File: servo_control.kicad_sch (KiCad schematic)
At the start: 23 parts, among them U9 PCA9685PW

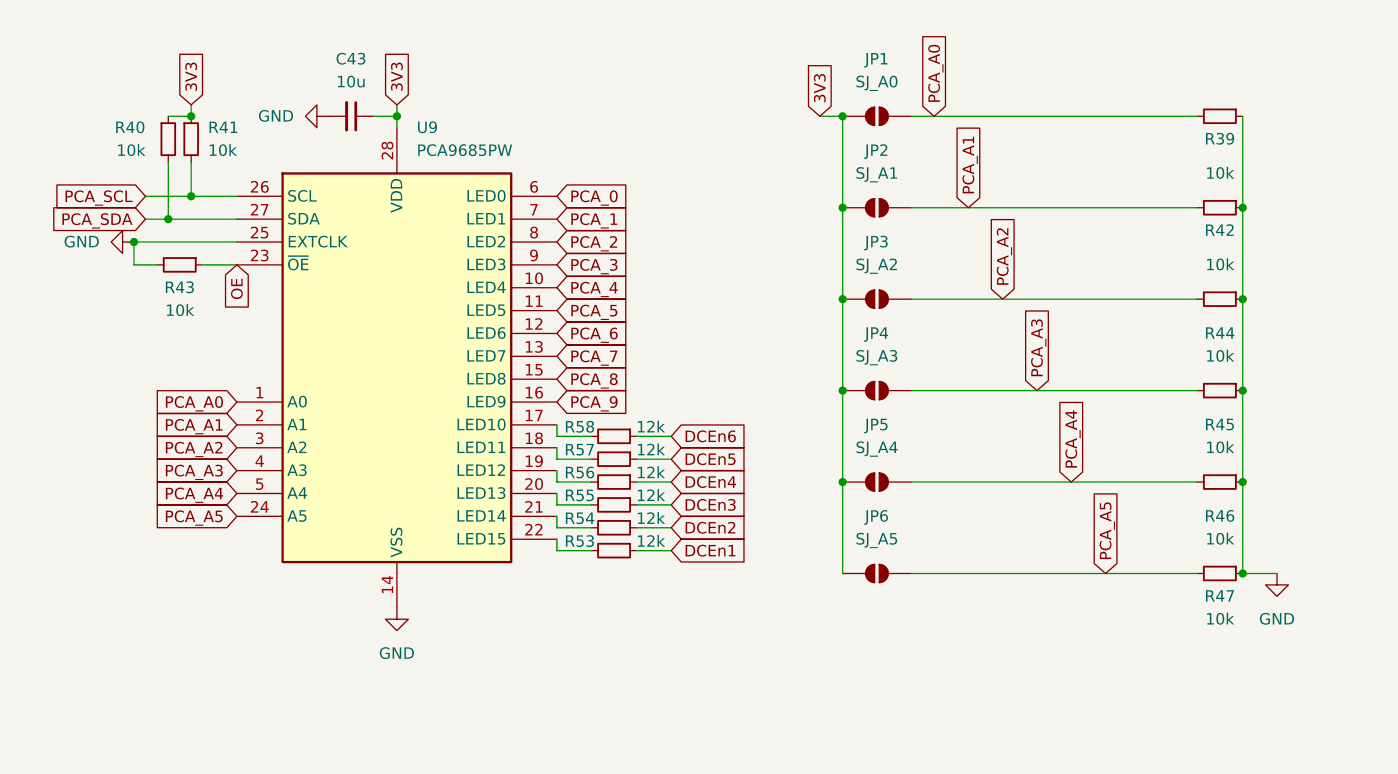
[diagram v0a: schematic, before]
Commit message: Visual Improvements
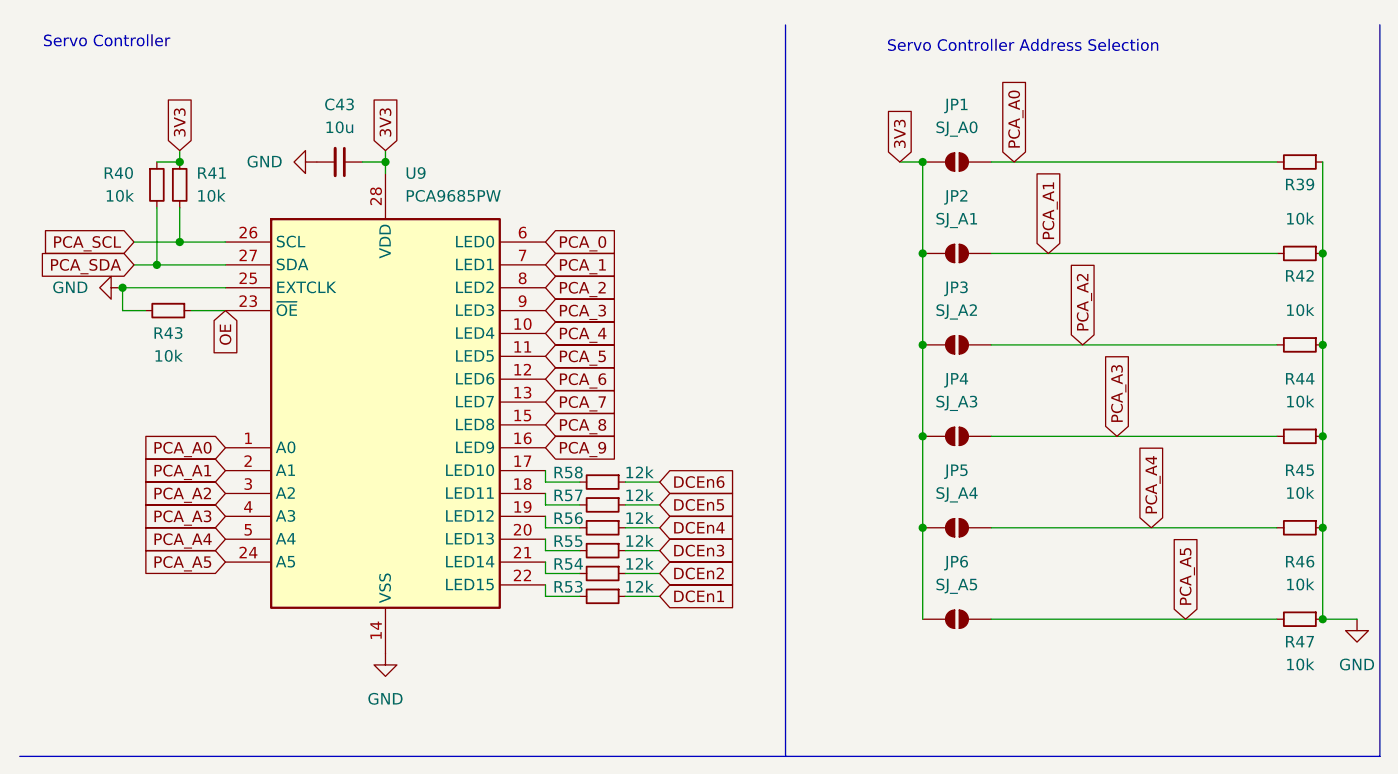
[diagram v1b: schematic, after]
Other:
- note added: "Servo Controller"
- note added: "Servo Controller Address Selection"
- moved on the sheet: C43, JP1, JP2, JP3, JP4, JP5, JP6, R39, R40, R41, R42, R43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

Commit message: schematic finished
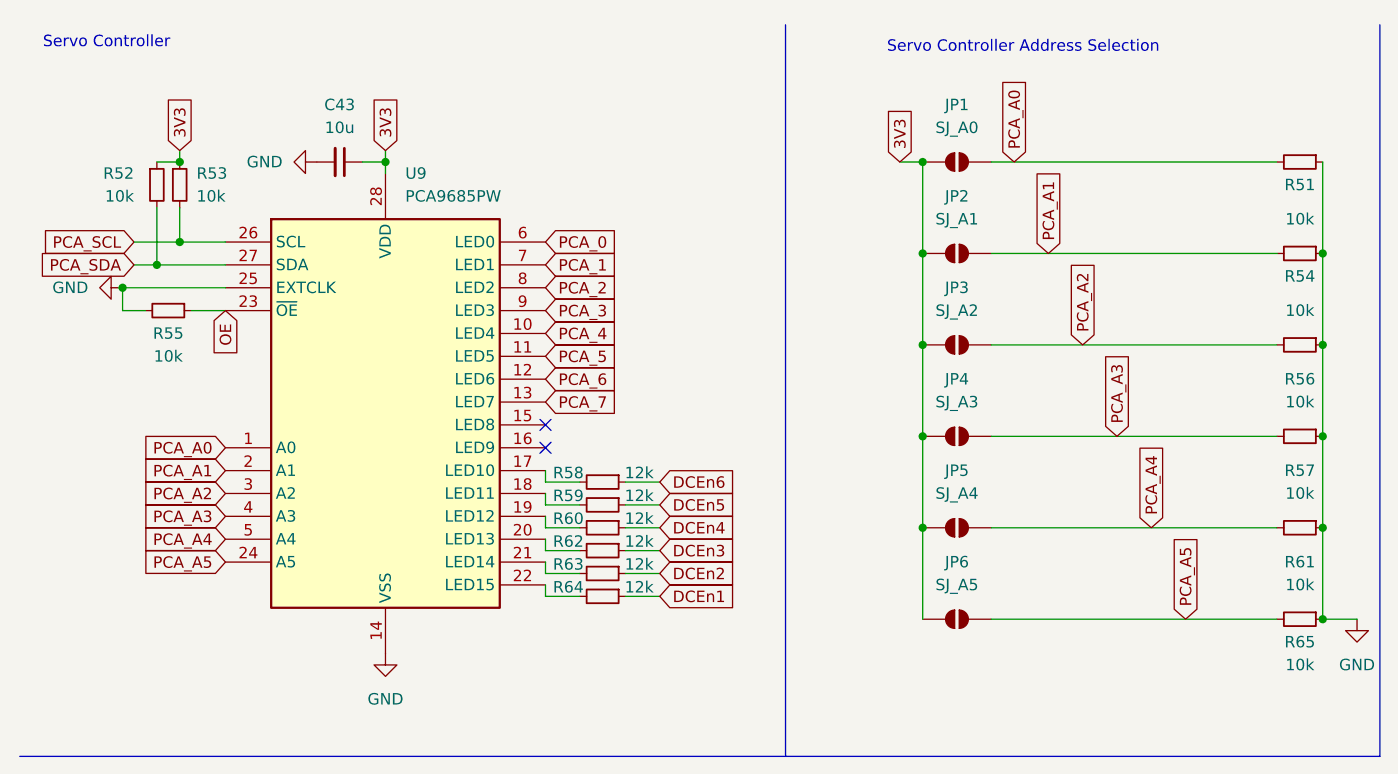
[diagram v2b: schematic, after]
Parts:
- renumbered R39 to R51, R40 to R52, R41 to R53, R42 to R54, R43 to R55, R44 to R56, R45 to R57, R57 to R59, R56 to R60, R46 to R61, R55 to R62, R54 to R63, R53 to R64, R47 to R65
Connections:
- net PCA_8: no longer names the net of U9.15 (LED8)
- net PCA_9: no longer names the net of U9.16 (LED9)
- no-connect marks 0 -> 2

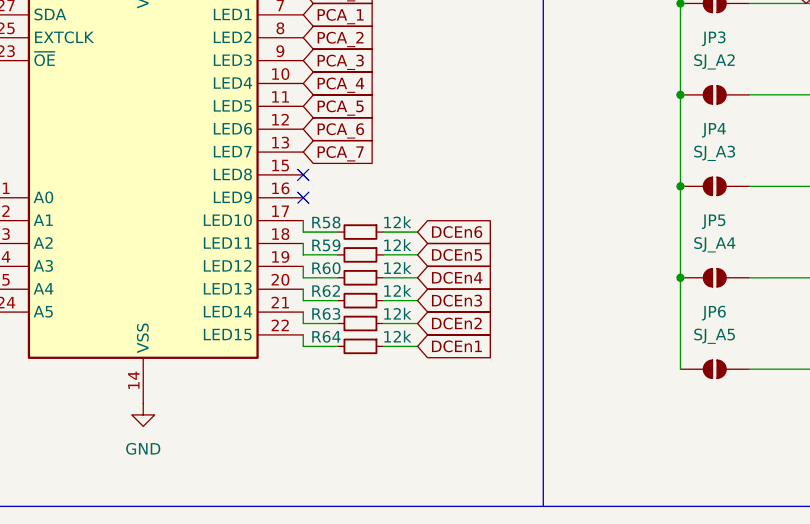
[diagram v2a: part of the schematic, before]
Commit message: Power Routing
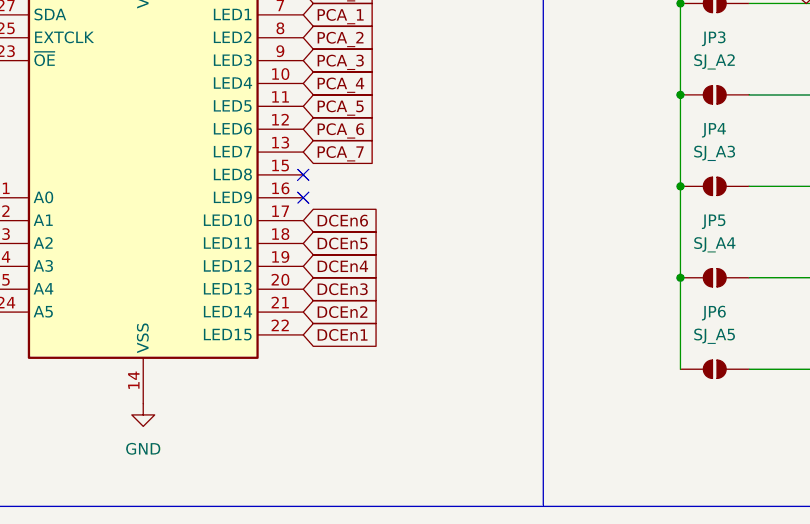
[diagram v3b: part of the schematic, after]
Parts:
- removed R58, R59, R60, R62, R63, R64: 12k, Resistor_SMD:R_0805_2012Metric, symbol Device:R_Small
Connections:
- net DCEn1: now also U9.22 (LED15)
- net DCEn2: now also U9.21 (LED14)
- net DCEn3: now also U9.20 (LED13)
- net DCEn4: now also U9.19 (LED12)
- net DCEn5: now also U9.18 (LED11)
- net DCEn6: now also U9.17 (LED10)

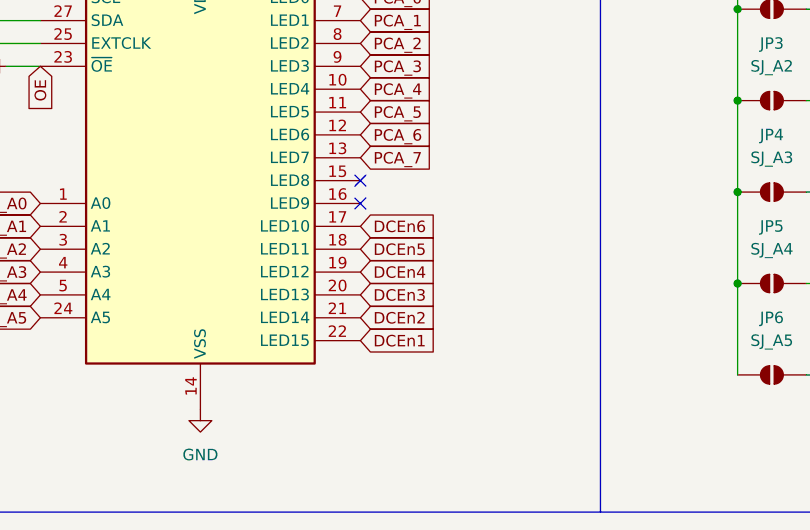
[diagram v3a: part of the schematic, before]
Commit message: yerleştirmeler devam
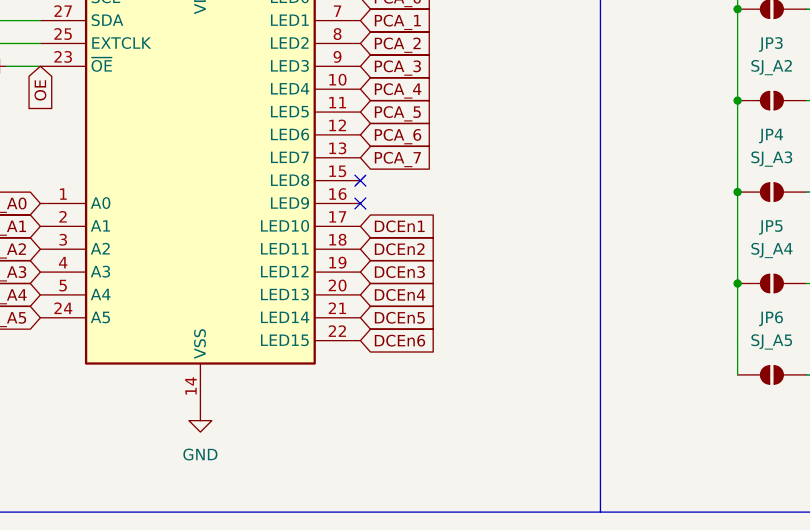
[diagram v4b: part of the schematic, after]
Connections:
- net DCEn1: now also U9.17 (LED10); no longer U9.22 (LED15)
- net DCEn2: now also U9.18 (LED11); no longer U9.21 (LED14)
- net DCEn3: now also U9.19 (LED12); no longer U9.20 (LED13)
- net DCEn4: now also U9.20 (LED13); no longer U9.19 (LED12)
- net DCEn5: now also U9.21 (LED14); no longer U9.18 (LED11)
- net DCEn6: now also U9.22 (LED15); no longer U9.17 (LED10)

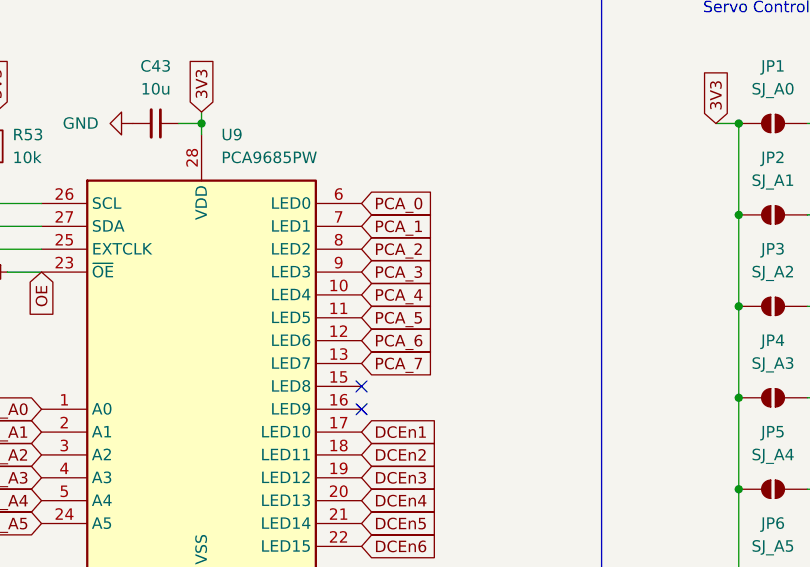
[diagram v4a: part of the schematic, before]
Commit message: Routing
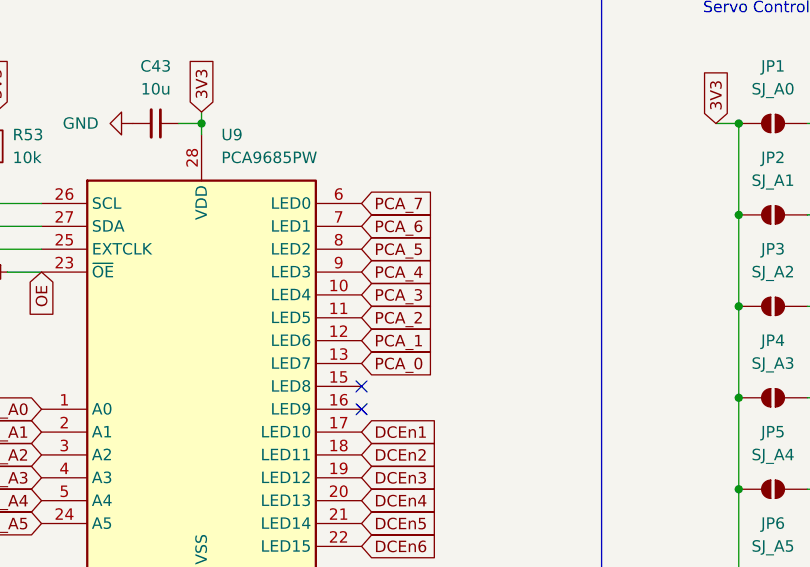
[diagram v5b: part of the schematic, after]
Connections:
- net PCA_0: now also U9.13 (LED7); no longer U9.6 (LED0)
- net PCA_1: now also U9.12 (LED6); no longer U9.7 (LED1)
- net PCA_2: now also U9.11 (LED5); no longer U9.8 (LED2)
- net PCA_3: now also U9.10 (LED4); no longer U9.9 (LED3)
- net PCA_4: now also U9.9 (LED3); no longer U9.10 (LED4)
- net PCA_5: now also U9.8 (LED2); no longer U9.11 (LED5)
- net PCA_6: now also U9.7 (LED1); no longer U9.12 (LED6)
- net PCA_7: now also U9.6 (LED0); no longer U9.13 (LED7)
